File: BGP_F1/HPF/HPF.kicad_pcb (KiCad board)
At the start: 2 copper layers, 30 x 24 mm, 15 parts, among them P1 CONN_01X05, P2 CONN_01X06, U1 MC33178

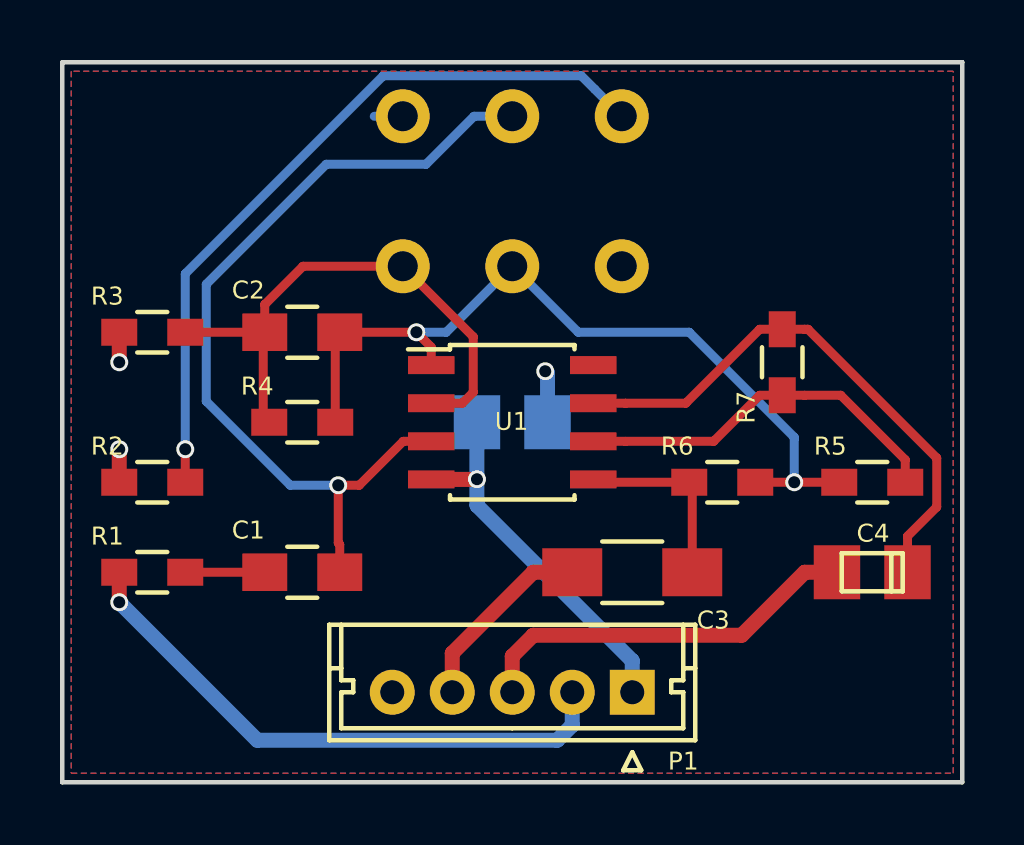
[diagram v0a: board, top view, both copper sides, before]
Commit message: Pot tinkering
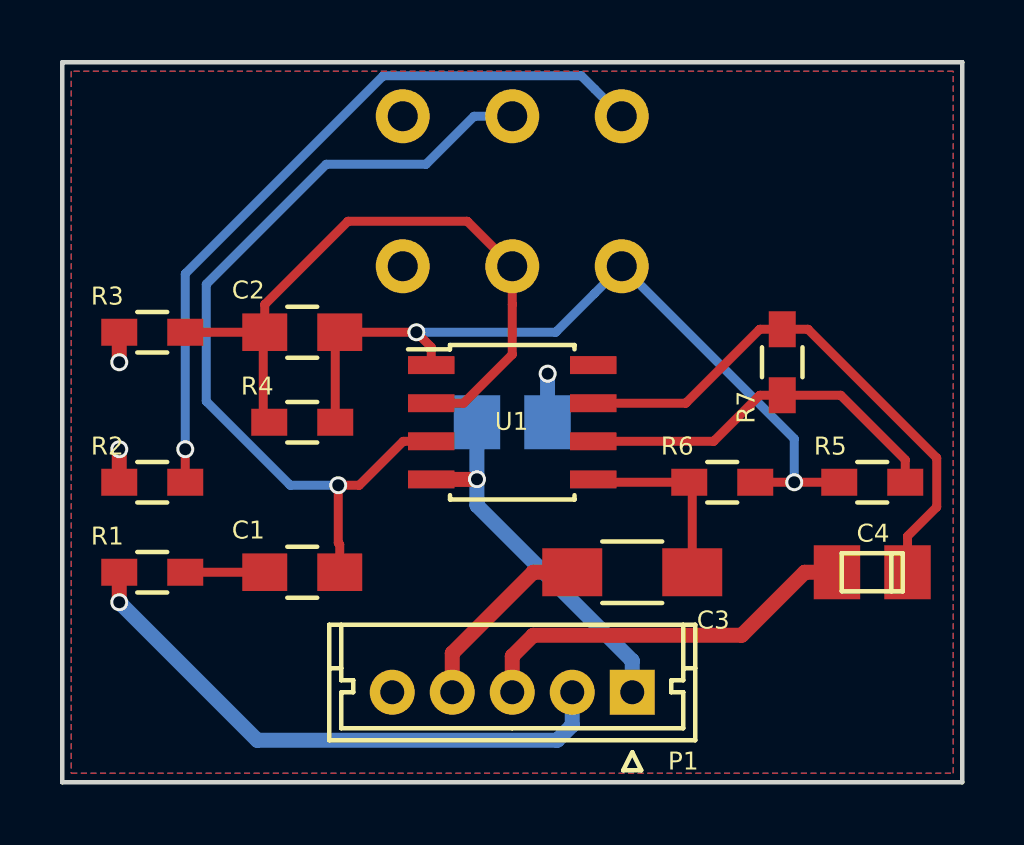
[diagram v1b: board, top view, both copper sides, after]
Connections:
- C2 pad 1: /VG_2 -> /VG_3
- C2 pad 2: /VG_1 -> /VG_2
- R3 pad 2: /VG_1 -> /VG_2
- R4 pad 1: /VG_2 -> /VG_3
- R4 pad 2: /VG_1 -> /VG_2
- R5 pad 2: /VG_2 -> /VG_3
- R6 pad 2: /VG_2 -> /VG_3
- U1 pad 1: /VG_2 -> /VG_3
- U1 pad 2: /VG_1 -> /VG_2
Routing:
- net /VG_3: track 0.00 -> 27.3 mm, vias 0 -> 2
- net /VG_1: track 18.5 -> 0.00 mm
- net /VG_2: track 27.2 -> 23.0 mm, vias 2 -> 0
- net /VF_1: track 0.95 -> 0.00 mm
